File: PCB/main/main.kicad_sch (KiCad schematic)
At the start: 4 parts, among them J1 Conn_01x33_Female, J2 Conn_01x33_Female, J3 Conn_01x33_Female, J4 Conn_01x33_Female

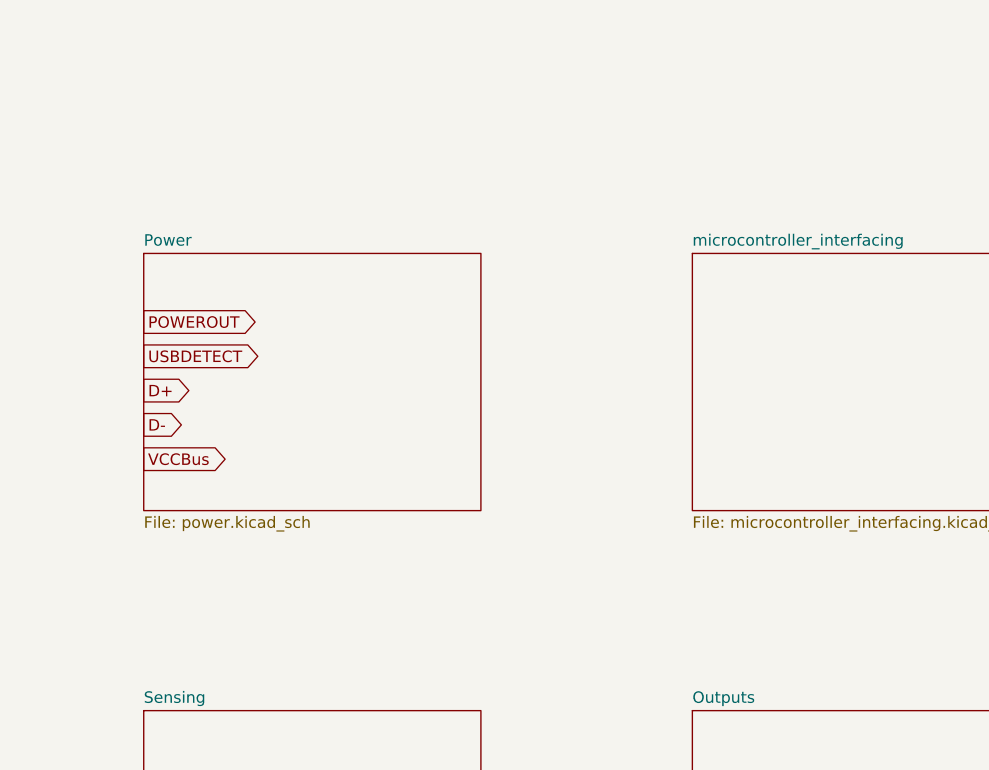
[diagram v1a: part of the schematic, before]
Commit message: Power v0.1, Sensing v0.1, uC Control v0.1, Simulations
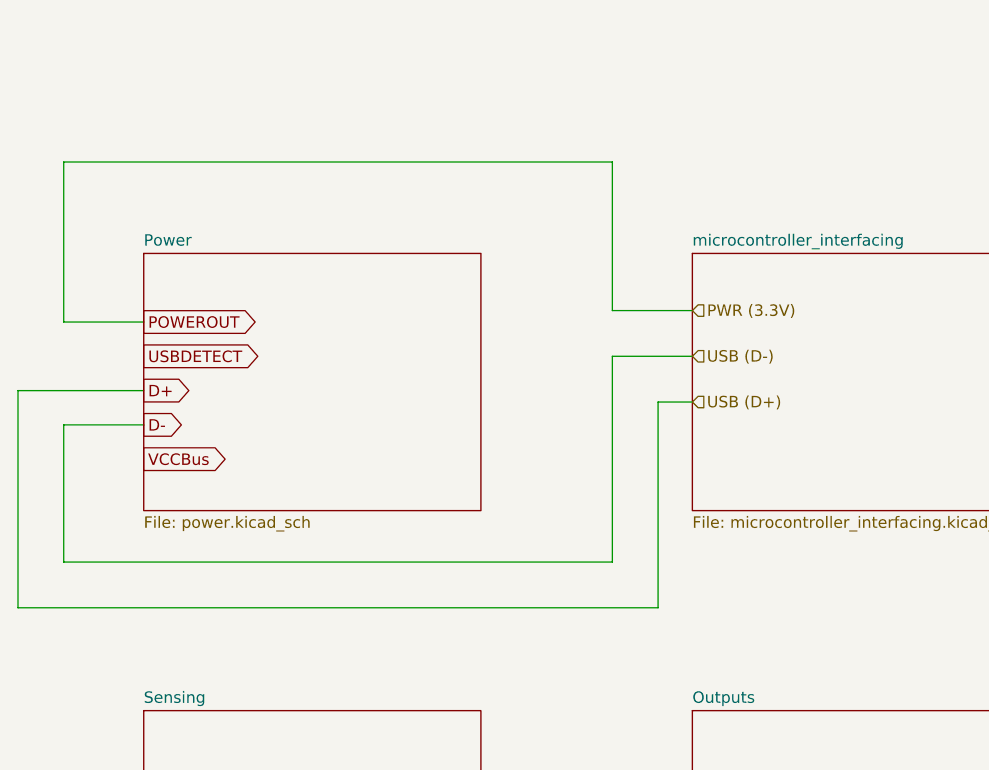
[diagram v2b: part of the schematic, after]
